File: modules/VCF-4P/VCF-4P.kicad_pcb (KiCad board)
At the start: 2 copper layers, 111.5 x 108.2 mm, 36 parts, among them J1 WQP-PJ398, J10 Conn_Front_Left_Top, J11 Conn_Back_Right_Top, J12 Conn_Front_Right, J13 Conn_Back_Left, J2 WQP-PJ398, J3 WQP-PJ398, J4 WQP-PJ398, J5 WQP-PJ398, J6 WQP-PJ398, J7 WQP-PJ398, J8 WQP-PJ398, J9 Conn_Eurorack_16, U3 TL072

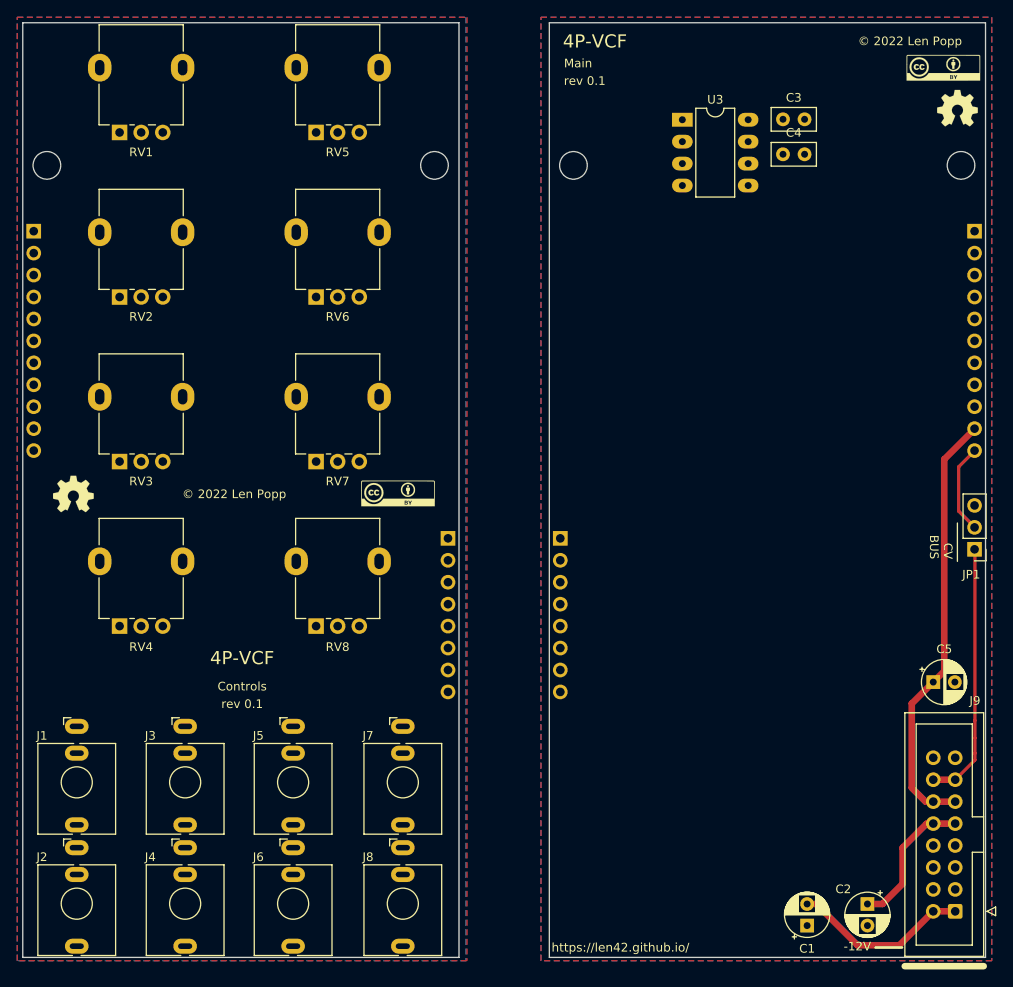
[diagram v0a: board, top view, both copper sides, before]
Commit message: VCF-4P: wip
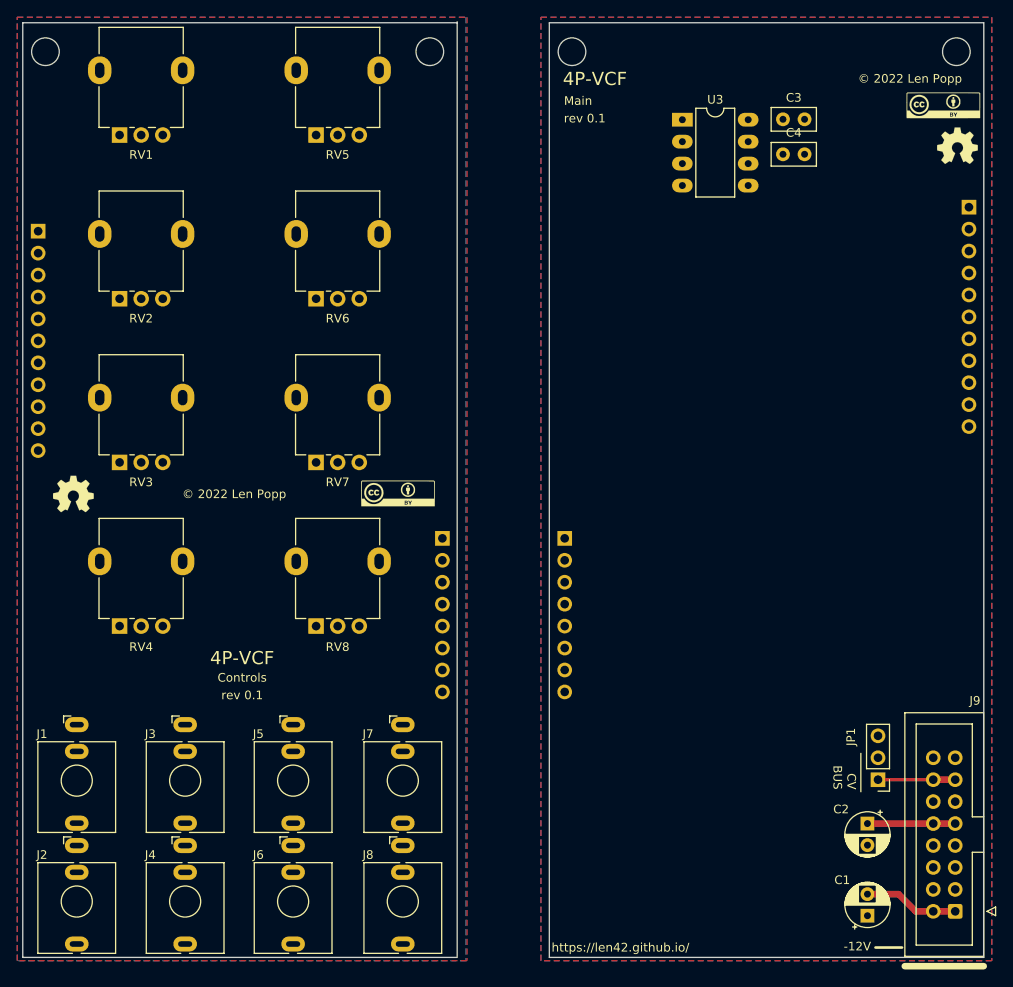
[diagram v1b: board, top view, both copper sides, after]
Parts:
- removed C5: 10U, -lmp-misc:CP_Radial_D5.0mm_P2.50mm
- moved JP1 28.9 mm to (195.5, 123.2)
- moved H2 13.2 mm to (143.6, 38.9)
- moved H4 13.2 mm to (204.6, 38.9)
- moved H1 13.2 mm to (99.1, 38.9)
- moved H3 13.2 mm to (160.1, 38.9)
- moved C2 9.31 mm to (194.3, 128.3)
- moved C1 7.08 mm to (194.3, 138.9)
- moved G1 4.34 mm to (203.1, 45.1)
- moved G3 4.34 mm to (204.7, 49.8)
- moved J11 2.85 mm to (206.1, 56.9)
- moved J12 0.65 mm to (145.1, 95.2)
- moved J13 0.51 mm to (159.3, 95.2)
- moved J10 0.51 mm to (98.3, 59.7)
- moved RV1 0.30 mm to (107.7, 48.6)
- moved RV5 0.30 mm to (130.5, 48.6)
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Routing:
- net +5V: track 50.4 -> 0.00 mm
- net Net-(J9-Pad13): track 30.2 -> 8.94 mm
- net IN-GATE-BUS: track 10.4 -> 0.00 mm
- net -12V: track 20.8 -> 11.0 mm
- net +12V: track 16.5 -> 10.2 mm
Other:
- board size 111.5 x 108.2 mm -> 111.3 x 108.3 mm
